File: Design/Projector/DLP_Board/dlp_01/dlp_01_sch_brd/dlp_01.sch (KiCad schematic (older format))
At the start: 0 parts

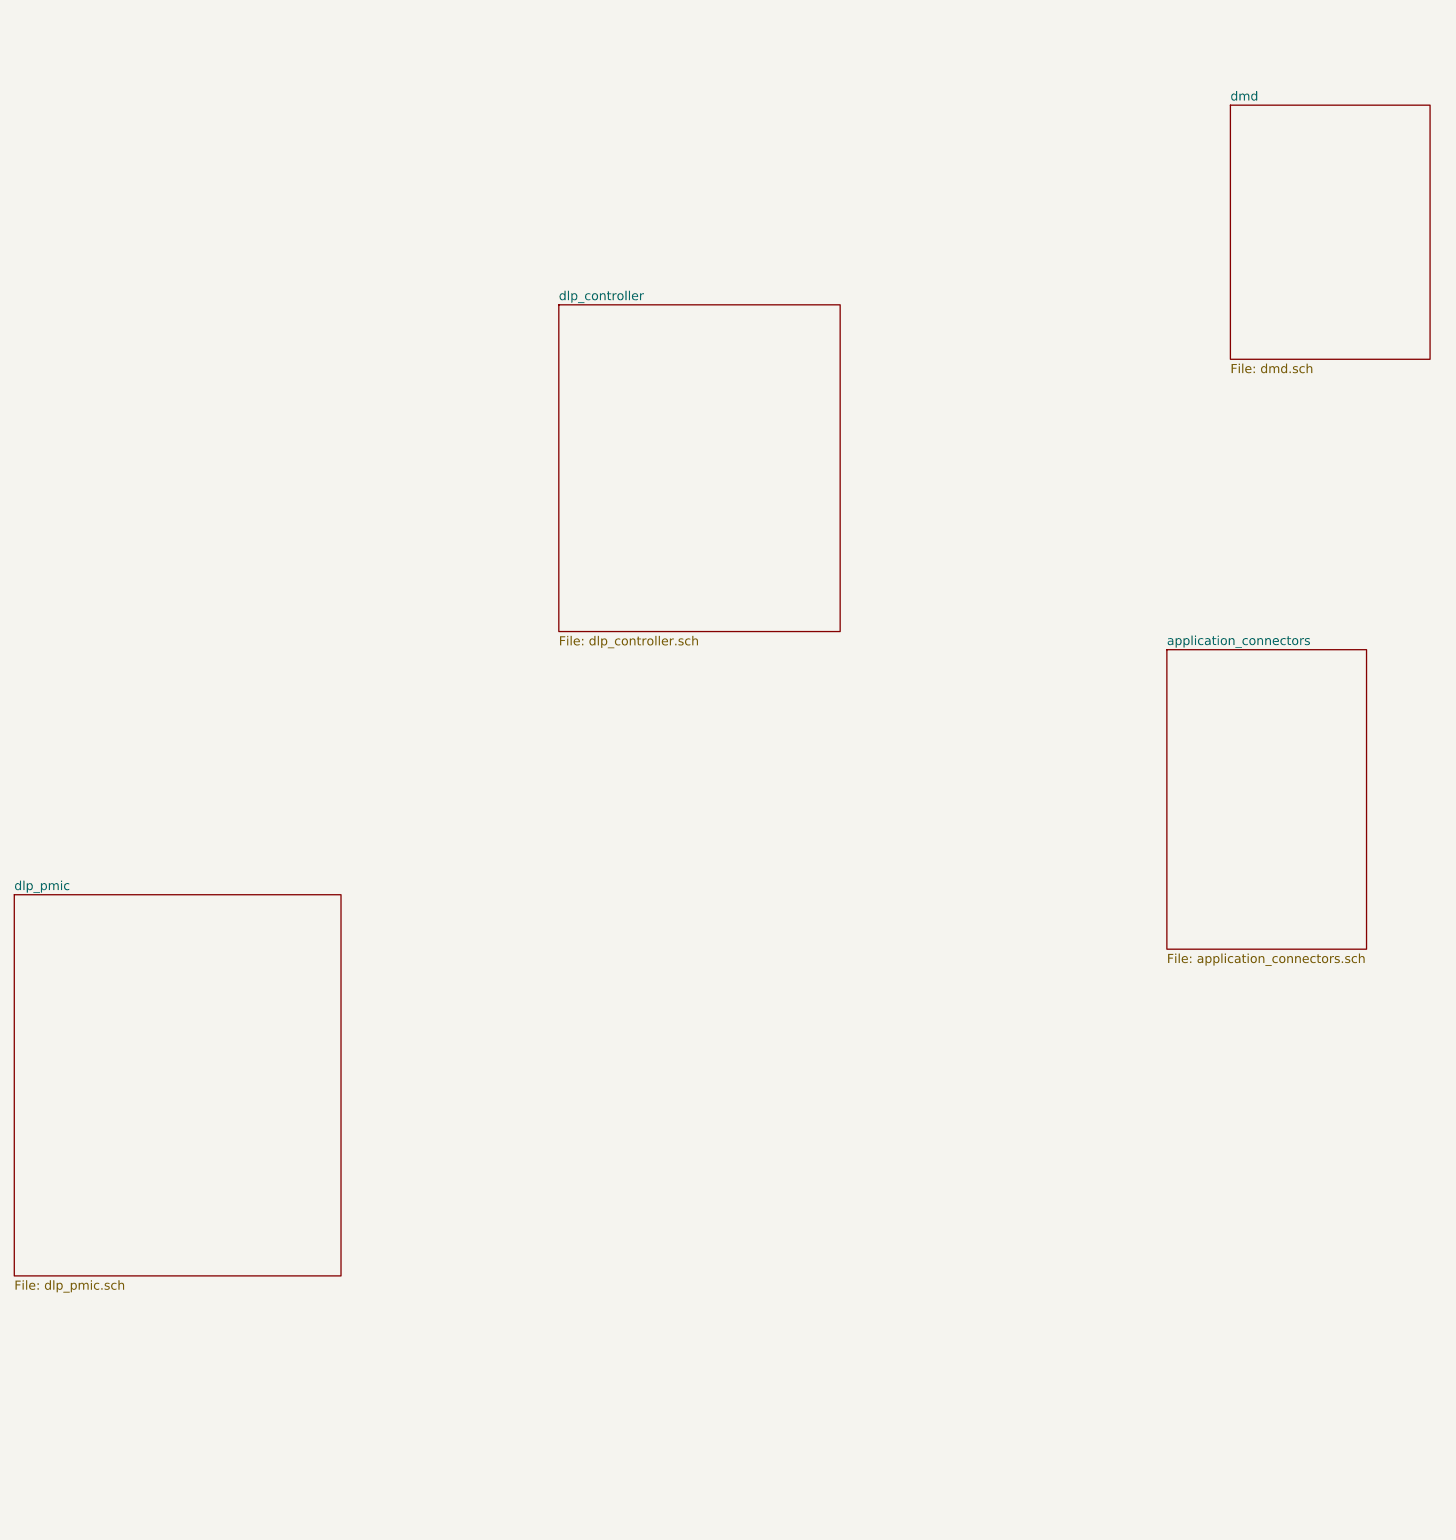
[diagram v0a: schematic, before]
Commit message: Ongoing updates the schematics
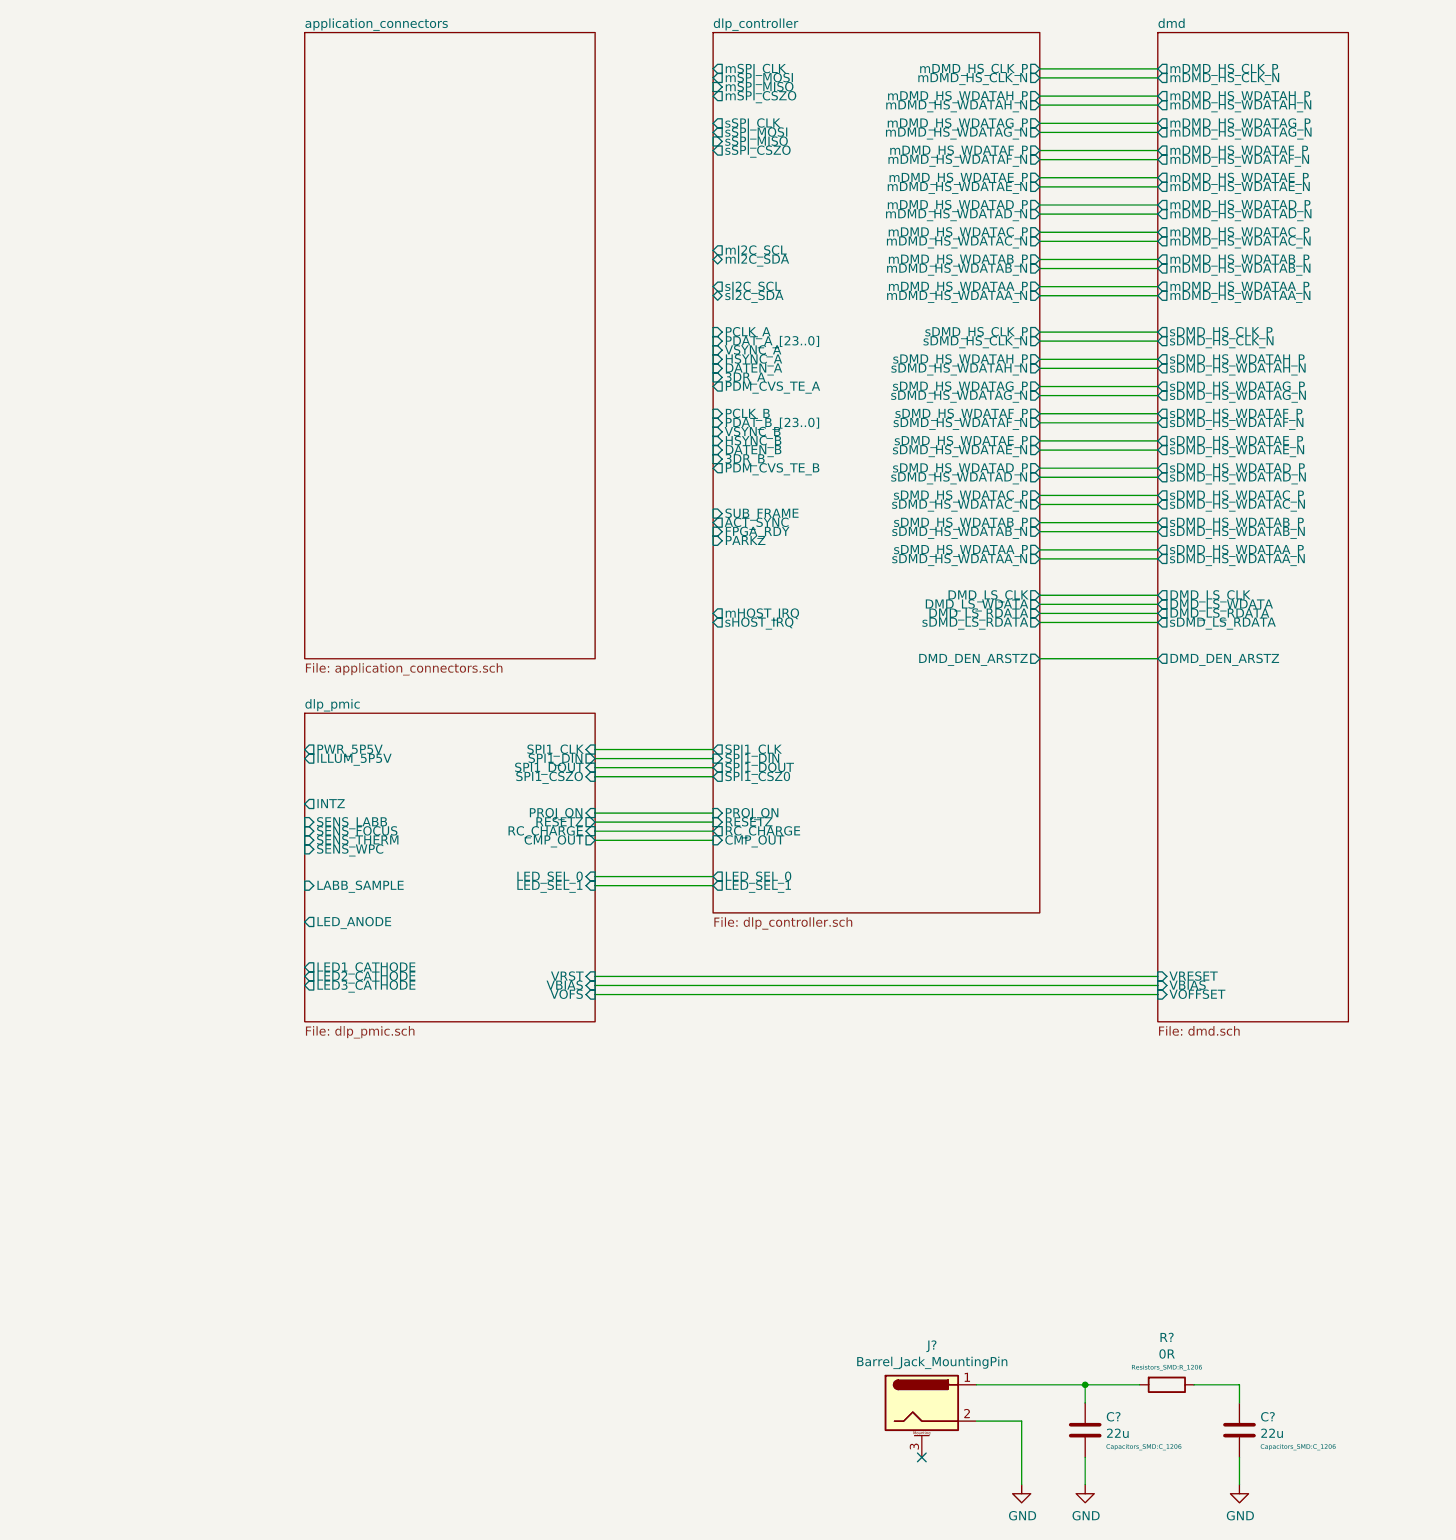
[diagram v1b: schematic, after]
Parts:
- added C? (x2): 22u, Capacitors_SMD:C_1206, symbol Device:C
- added J?: Barrel_Jack_MountingPin, Connectors:BARREL_JACK, symbol Connector:Barrel_Jack_MountingPin
- added R?: 0R, Resistors_SMD:R_1206, symbol Device:R
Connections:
- new net: C?.1, J?.1, R?.2
- new net: C?.1, R?.1
- new net GND: C?.2, C?.2, J?.2
- no-connect marks 0 -> 1

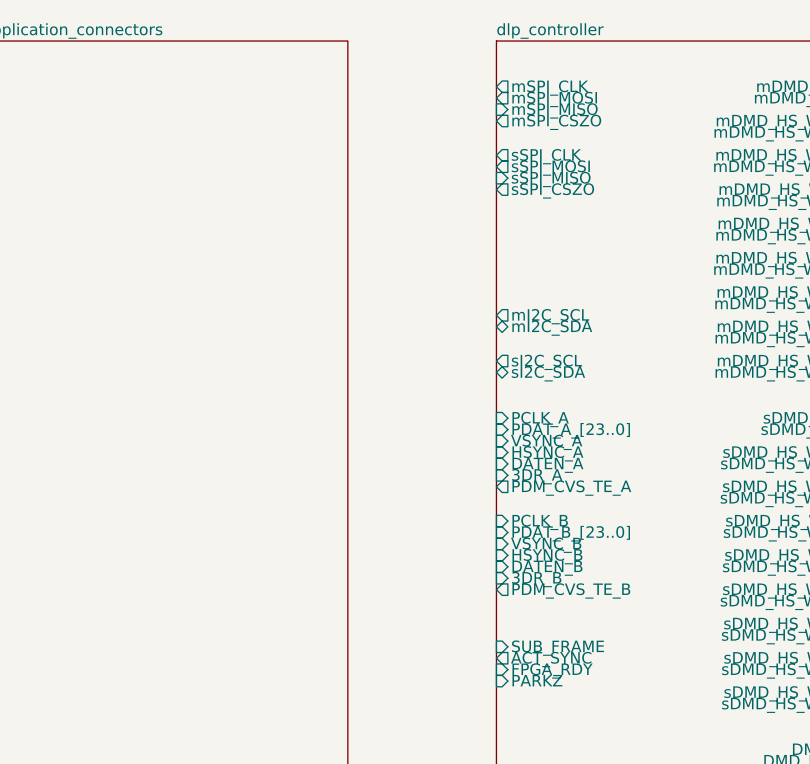
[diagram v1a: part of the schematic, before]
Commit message: More updates in the DLP board
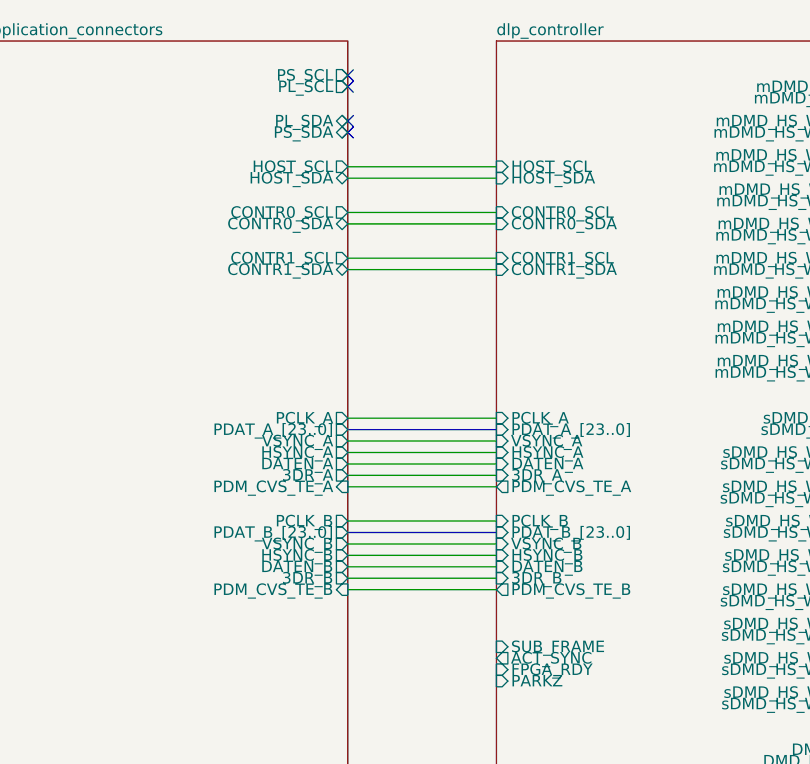
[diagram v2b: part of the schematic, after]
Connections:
- no-connect marks 1 -> 5
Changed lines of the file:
@@
 F64 "PDAT_A_[23..0]" I L 7700 4150 50
 F65 "3DR_A" I L 7700 4350 50
-F66 "mSPI_CLK" O L 7700 2650 50
-F67 "mSPI_MOSI" O L 7700 2700 50
-F68 "mSPI_CSZO" O L 7700 2800 50
-F69 "mSPI_MISO" I L 7700 2750 50
-F70 "mI2C_SCL" O L 7700 3650 50
-F71 "mI2C_SDA" B L 7700 3700 50
-F72 "mHOST_IRQ" O L 7700 5650 50
-F73 "CMP_OUT" I L 7700 6900 50
-F74 "LED_SEL_0" O L 7700 7100 50
-F75 "LED_SEL_1" O L 7700 7150 50
-F76 "sSPI_CLK" O L 7700 2950 50
-F77 "sSPI_MOSI" O L 7700 3000 50
-F78 "sSPI_CSZO" O L 7700 3100 50
-F79 "sSPI_MISO" I L 7700 3050 50
-F80 "sHOST_IRQ" O L 7700 5700 50
-F81 "sI2C_SCL" O L 7700 3850 50
-F82 "sI2C_SDA" B L 7700 3900 50
-F83 "PARKZ" I L 7700 5250 50
-F84 "RESETZ" I L 7700 6800 50
+F66 "mHOST_IRQ" O L 7700 5650 50
+F67 "CMP_OUT" I L 7700 6900 50
+F68 "LED_SEL_0" O L 7700 7100 50
+F69 "LED_SEL_1" O L 7700 7150 50
+F70 "sHOST_IRQ" O L 7700 5700 50
+F71 "PARKZ" I L 7700 5250 50
+F72 "RESETZ" I L 7700 6800 50
+F73 "HOST_SCL" I L 7700 3000 50
+F74 "HOST_SDA" I L 7700 3050 50
+F75 "CONTR0_SCL" I L 7700 3200 50
+F76 "CONTR0_SDA" I L 7700 3250 50
+F77 "CONTR1_SCL" I L 7700 3400 50
+F78 "CONTR1_SDA" I L 7700 3450 50
 $EndSheet
 $Sheet
@@
 F0 "application_connectors" 50
 F1 "application_connectors.sch" 50
+F2 "PCLK_B" O R 7050 4550 50
+F3 "VSYNC_B" O R 7050 4650 50
+F4 "HSYNC_B" O R 7050 4700 50
+F5 "DATEN_B" O R 7050 4750 50
+F6 "PDAT_B_[23..0]" O R 7050 4600 50
+F7 "3DR_B" O R 7050 4800 50
+F8 "PCLK_A" O R 7050 4100 50
+F9 "VSYNC_A" O R 7050 4200 50
+F10 "HSYNC_A" O R 7050 4250 50
+F11 "DATEN_A" O R 7050 4300 50
+F12 "PDAT_A_[23..0]" O R 7050 4150 50
+F13 "3DR_A" O R 7050 4350 50
+F14 "PDM_CVS_TE_B" I R 7050 4850 50
+F15 "PDM_CVS_TE_A" I R 7050 4400 50
+F16 "HOST_SCL" O R 7050 3000 50
+F17 "HOST_SDA" B R 7050 3050 50
+F18 "CONTR0_SCL" O R 7050 3200 50
+F19 "CONTR0_SDA" B R 7050 3250 50
+F20 "CONTR1_SDA" B R 7050 3450 50
+F21 "CONTR1_SCL" O R 7050 3400 50
+F22 "PS_SCL" O R 7050 2600 50
+F23 "PL_SCL" O R 7050 2650 50
+F24 "PL_SDA" B R 7050 2800 50
+F25 "PS_SDA" B R 7050 2850 50
 $EndSheet
 Wire Wire Line
@@
 Wire Wire Line
 	7050 7750 10150 7750
+Wire Wire Line
+	7050 4100 7700 4100
+Wire Wire Line
+	7050 4200 7700 4200
+Wire Bus Line
+	7050 4150 7700 4150
+Wire Wire Line
+	7050 4250 7700 4250
+Wire Wire Line
+	7050 4300 7700 4300
+Wire Wire Line
+	7050 4350 7700 4350
+Wire Wire Line
+	7050 4400 7700 4400
+Wire Wire Line
+	7050 4550 7700 4550
+Wire Bus Line
+	7050 4600 7700 4600
+Wire Wire Line
+	7050 4650 7700 4650
+Wire Wire Line
+	7050 4700 7700 4700
+Wire Wire Line
+	7050 4750 7700 4750
+Wire Wire Line
+	7050 4800 7700 4800
+Wire Wire Line
+	7050 4850 7700 4850
+NoConn ~ 7050 2600
+NoConn ~ 7050 2650
+NoConn ~ 7050 2800
+NoConn ~ 7050 2850
+Wire Wire Line
+	7050 3000 7700 3000
+Wire Wire Line
+	7700 3050 7050 3050
+Wire Wire Line
+	7050 3200 7700 3200
+Wire Wire Line
+	7700 3250 7050 3250
+Wire Wire Line
+	7050 3400 7700 3400
+Wire Wire Line
+	7700 3450 7050 3450
 $EndSCHEMATC
